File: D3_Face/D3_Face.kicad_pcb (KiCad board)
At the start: 2 copper layers, 100 x 70 mm, 31 parts, among them J1 Conn_01x05_Male, U1 MAX7219, U2 MAX7219, U3 MAX7219, U4 MAX7219, U5 MAX7219, U6 MAX7219

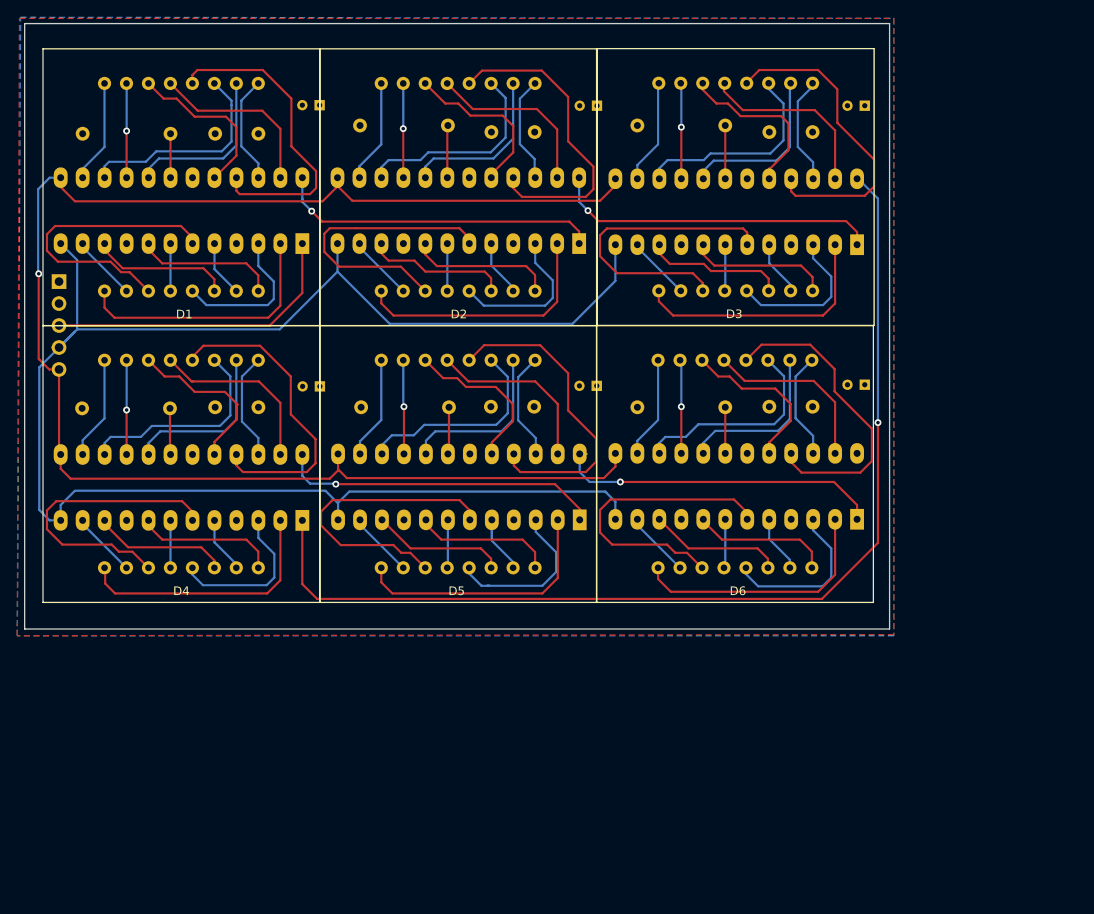
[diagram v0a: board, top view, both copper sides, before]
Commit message: Create D3_Board
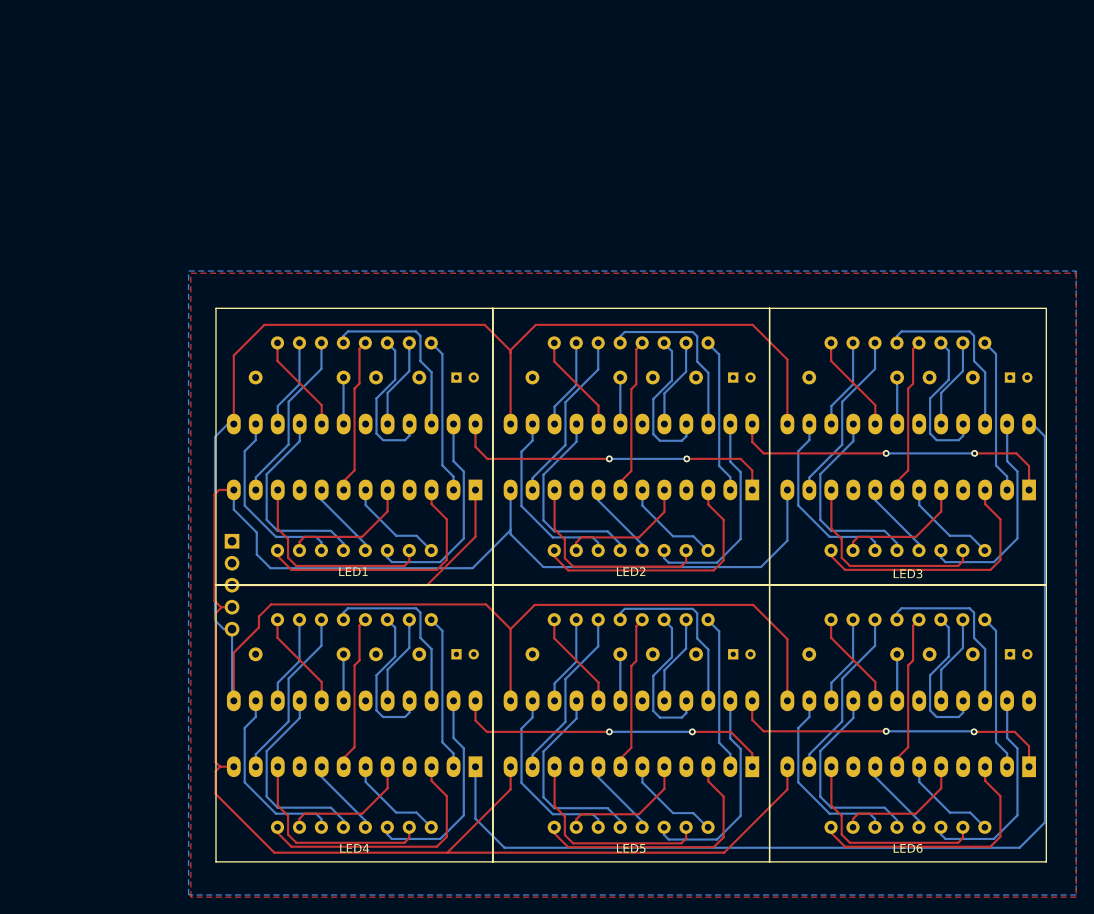
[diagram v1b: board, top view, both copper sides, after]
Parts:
- removed D1, D2, D3, D4, D5, D6: Matrix_LED_8x8, D3_Face:Matrix_LED_8x8
- added LED1: Matrix_LED_8x8, D3_Face:Matrix_LED_8x8, F.Cu at (120.0, 80.0)
- added LED2: Matrix_LED_8x8, D3_Face:Matrix_LED_8x8, F.Cu at (152.0, 80.0)
- added LED3: Matrix_LED_8x8, D3_Face:Matrix_LED_8x8, F.Cu at (184.0, 80.0)
- added LED4: Matrix_LED_8x8, D3_Face:Matrix_LED_8x8, F.Cu at (120.0, 112.0)
- added LED5: Matrix_LED_8x8, D3_Face:Matrix_LED_8x8, F.Cu at (152.0, 112.0)
- added LED6: Matrix_LED_8x8, D3_Face:Matrix_LED_8x8, F.Cu at (184.0, 112.0)
- moved C12 57.0 mm to (195.8, 104.0), turned to 0 degrees
- moved J1 36.1 mm to (105.9, 90.9)
- moved C6 35.6 mm to (195.8, 72.0), turned to 0 degrees
- moved R2 35.3 mm to (140.6, 72.0)
- moved R3 35.3 mm to (172.6, 72.0)
- moved C4 35.2 mm to (131.8, 72.0), turned to 0 degrees
- moved C5 35.1 mm to (163.8, 72.0), turned to 0 degrees
- moved U6 34.8 mm to (198.0, 117.0)
- moved U5 34.8 mm to (166.0, 117.0)
- moved U1 34.8 mm to (134.0, 85.0)
- moved U2 34.8 mm to (166.0, 85.0)
- moved U4 34.8 mm to (134.0, 117.0)
- moved R4 34.8 mm to (108.6, 104.0)
- moved R6 34.8 mm to (172.6, 104.0)
- moved C10 34.8 mm to (131.8, 104.0), turned to 0 degrees
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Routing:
- net CLK: track 178.4 -> 222.5 mm, vias 1 -> 0
- net CS: track 189.0 -> 217.2 mm
- net Net-(LED3-Pad8): track 35.4 -> 11.5 mm
- net Net-(LED5-Pad8): track 35.0 -> 11.5 mm
- net Net-(LED6-Pad8): track 35.0 -> 11.5 mm
- net Net-(LED4-Pad8): track 34.5 -> 11.5 mm
- net Net-(LED1-Pad8): track 34.0 -> 11.5 mm
- net Net-(LED2-Pad8): track 33.9 -> 11.5 mm
- net Net-(LED3-Pad11): track 38.0 -> 17.5 mm
- net Net-(LED5-Pad11): track 36.7 -> 17.5 mm
- net Net-(LED1-Pad11): track 36.7 -> 17.5 mm
- net Net-(LED2-Pad11): track 36.5 -> 17.5 mm
- net Net-(LED4-Pad11): track 36.1 -> 17.5 mm
- net Net-(LED6-Pad11): track 36.0 -> 17.5 mm
- net Net-(LED1-Pad15): track 25.5 -> 10.4 mm
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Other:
- board outline removed
